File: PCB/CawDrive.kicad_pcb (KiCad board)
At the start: 4 copper layers, 50 x 42 mm, 112 parts, among them CN2 WAFER-SH1.0-6PWB, CN3 WAFER-SH1.0-4PWB, Q1 NMOS, Q10 TPH3R704PL, Q11 TPH3R704PL, Q12 TPH3R704PL, Q7 TPH3R704PL, Q8 TPH3R704PL, Q9 TPH3R704PL, U1 TJA1051T/3/1J, U10 WAFER-SH1.0-2PWB, U11 WAFER-SH1.0-2PWB, U12 WAFER-SH1.0-2PWB, U2 TLV76733DRVR, U5 WAFER-SH1.0-2PWB, U6 WAFER-SH1.0-2PWB, U7 DRV8323RSRGZR, U8 STM32F446RETx, U9 MT6835GT-STD, X1 CSTNE16M0V530000R0

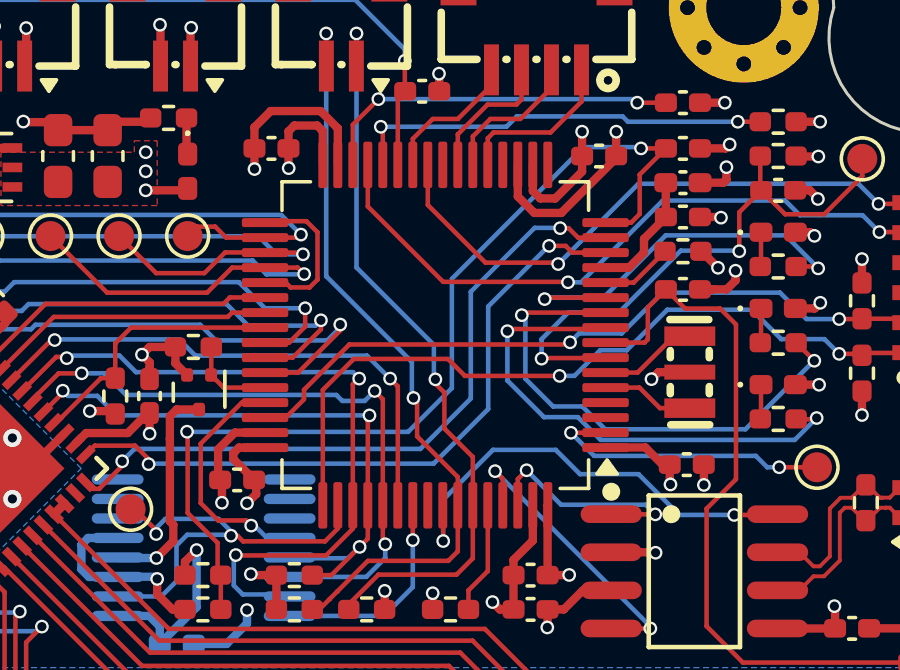
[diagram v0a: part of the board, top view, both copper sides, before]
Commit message: refactor: 将符号表和封装导出到项目中
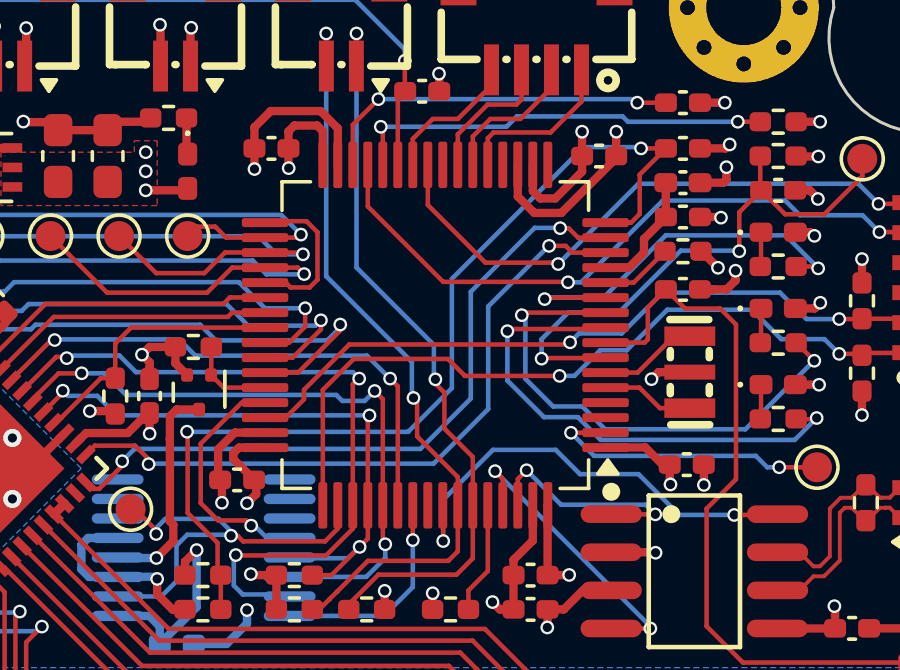
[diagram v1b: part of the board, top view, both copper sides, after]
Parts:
- C1, C10, C11, C12, C13, C14, C17, C18, C19, C2, C27, C3, C31, C32, C4, C5, C6, C7, C9: footprint Capacitor_SMD:C_0402_1005Metric_Pad0.74x0.62mm_HandSolder -> Library:C_0402_1005Metric_Pad0.74x0.62mm_HandSolder
- C15, C16, C28, C33, C34, C35: footprint Capacitor_SMD:C_0603_1608Metric_Pad1.08x0.95mm_HandSolder -> Library:C_0603_1608Metric_Pad1.08x0.95mm_HandSolder
- C20, C21, C22, C23, C24, C25, C26, C29, C30, C36, C37, C38: footprint Capacitor_SMD:C_1206_3216Metric_Pad1.33x1.80mm_HandSolder -> Library:C_1206_3216Metric_Pad1.33x1.80mm_HandSolder
- CN2: footprint Rick_Connector:CONN-SMD_6P-P1.00_XUNPU_WAFER-SH1.0-6PWB -> Library:CONN-SMD_6P-P1.00_XUNPU_WAFER-SH1.0-6PWB
- CN3: footprint Rick_Connector:CONN-SMD_4P-P1.00_WAFER-SH1.0-4PWB -> Library:CONN-SMD_4P-P1.00_WAFER-SH1.0-4PWB
- D1, D2, D4, D6: footprint LED_SMD:LED_0402_1005Metric_Pad0.77x0.64mm_HandSolder -> Library:LED_0402_1005Metric_Pad0.77x0.64mm_HandSolder
- D3: footprint Diode_SMD:D_SOD-123 -> Library:D_SOD-123
- G***: footprint Rick_Logo:guaik_logo_black_7x7 -> Library:guaik_logo_black_7x7
- H1, H2, H3, H4: footprint MountingHole:MountingHole_2.5mm_Pad_Via -> Library:MountingHole_2.5mm_Pad_Via
- H5, H6, H7, H8, H9: footprint CawDrive_Connector:POWER_PAD -> Library:POWER_PAD
- L1: footprint Inductor_SMD:L_0402_1005Metric_Pad0.77x0.64mm_HandSolder -> Library:L_0402_1005Metric_Pad0.77x0.64mm_HandSolder
- L2: footprint Rick_Inductor:LQH5BPB220MT0L_IND-SMD_L5.0-W5.0 -> Library:LQH5BPB220MT0L_IND-SMD_L5.0-W5.0
- Q1: footprint Package_TO_SOT_SMD:SOT-723 -> Library:SOT-723
- Q10, Q11, Q12, Q7, Q8, Q9: footprint Rick_MOSFET:TPHR8504PL,L1Q -> Library:TPHR8504PL,L1Q
- R1, R10, R11, R12, R13, R14, R15, R16, R17, R2, R20, R21, R22, R23, R24, R25, R26, R3, R4, R5, R6, R7, R8, R9: footprint Resistor_SMD:R_0402_1005Metric_Pad0.72x0.64mm_HandSolder -> Library:R_0402_1005Metric_Pad0.72x0.64mm_HandSolder
- R18, R19: footprint Resistor_SMD:R_1210_3225Metric_Pad1.30x2.65mm_HandSolder -> Library:R_1210_3225Metric_Pad1.30x2.65mm_HandSolder
- TP1, TP2, TP3, TP4, TP5, TP6, TP7, TP8, TP9: footprint TestPoint:TestPoint_Pad_D1.0mm -> Library:TestPoint_Pad_D1.0mm
- TV1: footprint Rick_Diode:SMAJ36CA_TR13_SMA(DO-214AC) -> Library:SMAJ36CA_TR13_SMA(DO-214AC)
- U1: footprint Rick_CAN:TJA1051T31J_SOIC-8_L4.9-W3.9-P1.27-LS6.0-BL -> Library:TJA1051T31J_SOIC-8_L4.9-W3.9-P1.27-LS6.0-BL
- U10, U11, U12, U5, U6: footprint Rick_Connector:CONN-SMD_2P-P1.00_XUNPU_WAFER-SH1.0-2PWB -> Library:CONN-SMD_2P-P1.00_XUNPU_WAFER-SH1.0-2PWB
- U2: footprint Rick_Regulator_Linear:TLV76733DRVR_SON65P200X200X80-7N -> Library:TLV76733DRVR_SON65P200X200X80-7N
- U7: footprint Rick_Drive:DRV8323RS_QFN-48-EP(7x7) -> Library:DRV8323RS_QFN-48-EP(7x7)
- U8: footprint Package_QFP:LQFP-64_10x10mm_P0.5mm -> Library:LQFP-64_10x10mm_P0.5mm
- U9: footprint Rick_Sensor:MT6835GT-STD -> Library:MT6835GT-STD
- X1: footprint Rick_Crystal:Crystal_SMD3213-3P -> Library:Crystal_SMD3213-3P
- kibuzzard-692C9A5B: footprint kibuzzard-692C9A5B -> Library:kibuzzard-692C9A5B
- kibuzzard-692C9AA1: footprint kibuzzard-692C9AA1 -> Library:kibuzzard-692C9AA1

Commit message: fix(CawDrive.kicad_pcb): 修复丝印相关的warning
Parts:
- C1, C10, C11, C12, C13, C14, C17, C18, C19, C2, C27, C3, C31, C32, C4, C5, C6, C7, C9: footprint Library:C_0402_1005Metric_Pad0.74x0.62mm_HandSolder -> Capacitor_SMD:C_0402_1005Metric_Pad0.74x0.62mm_HandSolder
- C15, C16, C28, C33, C34, C35: footprint Library:C_0603_1608Metric_Pad1.08x0.95mm_HandSolder -> Capacitor_SMD:C_0603_1608Metric_Pad1.08x0.95mm_HandSolder
- C20, C21, C22, C23, C24, C25, C26, C29, C30, C36, C37, C38: footprint Library:C_1206_3216Metric_Pad1.33x1.80mm_HandSolder -> Capacitor_SMD:C_1206_3216Metric_Pad1.33x1.80mm_HandSolder
- CN2: footprint Library:CONN-SMD_6P-P1.00_XUNPU_WAFER-SH1.0-6PWB -> Rick_Connector:CONN-SMD_6P-P1.00_XUNPU_WAFER-SH1.0-6PWB
- CN3: footprint Library:CONN-SMD_4P-P1.00_WAFER-SH1.0-4PWB -> Rick_Connector:CONN-SMD_4P-P1.00_WAFER-SH1.0-4PWB
- D1, D2, D4, D6: footprint Library:LED_0402_1005Metric_Pad0.77x0.64mm_HandSolder -> LED_SMD:LED_0402_1005Metric_Pad0.77x0.64mm_HandSolder
- D3: footprint Library:D_SOD-123 -> Diode_SMD:D_SOD-123
- H1, H2, H3, H4: footprint Library:MountingHole_2.5mm_Pad_Via -> MountingHole:MountingHole_2.5mm_Pad_Via
- H5, H6, H7, H8, H9: footprint Library:POWER_PAD -> CawDrive_Connector:POWER_PAD
- L1: footprint Library:L_0402_1005Metric_Pad0.77x0.64mm_HandSolder -> Inductor_SMD:L_0402_1005Metric_Pad0.77x0.64mm_HandSolder
- L2: footprint Library:LQH5BPB220MT0L_IND-SMD_L5.0-W5.0 -> Rick_Inductor:LQH5BPB220MT0L_IND-SMD_L5.0-W5.0
- Q1: footprint Library:SOT-723 -> Package_TO_SOT_SMD:SOT-723
- Q10, Q11, Q12, Q7, Q8, Q9: footprint Library:TPHR8504PL,L1Q -> Rick_MOSFET:TPHR8504PL,L1Q
- R1, R10, R11, R12, R13, R14, R15, R16, R17, R2, R20, R21, R22, R23, R24, R25, R26, R3, R4, R5, R6, R7, R8, R9: footprint Library:R_0402_1005Metric_Pad0.72x0.64mm_HandSolder -> Resistor_SMD:R_0402_1005Metric_Pad0.72x0.64mm_HandSolder
- R18, R19: footprint Library:R_1210_3225Metric_Pad1.30x2.65mm_HandSolder -> Resistor_SMD:R_1210_3225Metric_Pad1.30x2.65mm_HandSolder
- TP1, TP2, TP3, TP4, TP5, TP6, TP7, TP8, TP9: footprint Library:TestPoint_Pad_D1.0mm -> TestPoint:TestPoint_Pad_D1.0mm
- TV1: footprint Library:SMAJ36CA_TR13_SMA(DO-214AC) -> Rick_Diode:SMAJ36CA_TR13_SMA(DO-214AC)
- U1: footprint Library:TJA1051T31J_SOIC-8_L4.9-W3.9-P1.27-LS6.0-BL -> Rick_CAN:TJA1051T31J_SOIC-8_L4.9-W3.9-P1.27-LS6.0-BL
- U10, U11, U12, U5, U6: footprint Library:CONN-SMD_2P-P1.00_XUNPU_WAFER-SH1.0-2PWB -> Rick_Connector:CONN-SMD_2P-P1.00_XUNPU_WAFER-SH1.0-2PWB
- U2: footprint Library:TLV76733DRVR_SON65P200X200X80-7N -> Rick_Regulator_Linear:TLV76733DRVR_SON65P200X200X80-7N
- U7: footprint Library:DRV8323RS_QFN-48-EP(7x7) -> Rick_Drive:DRV8323RS_QFN-48-EP(7x7)
- U8: footprint Library:LQFP-64_10x10mm_P0.5mm -> Package_QFP:LQFP-64_10x10mm_P0.5mm
- U9: footprint Library:MT6835GT-STD -> Rick_Sensor:MT6835GT-STD
- X1: footprint Library:Crystal_SMD3213-3P -> Rick_Crystal:Crystal_SMD3213-3P
